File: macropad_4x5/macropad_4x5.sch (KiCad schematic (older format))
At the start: 41 parts

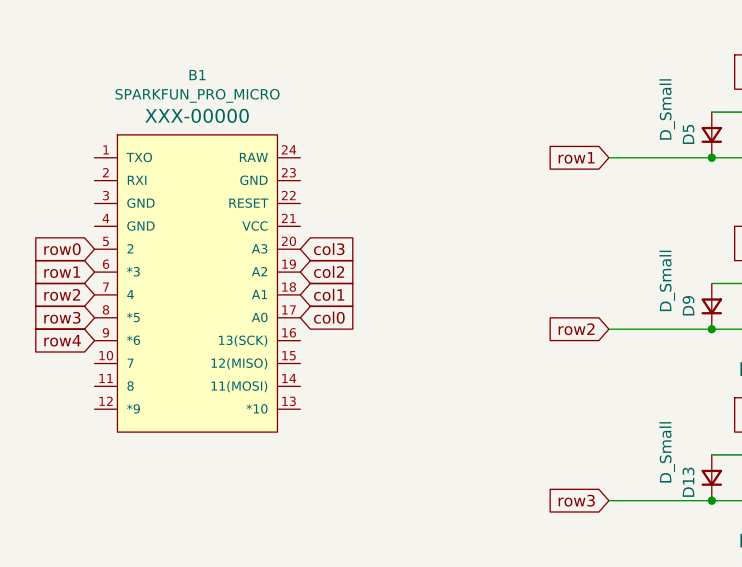
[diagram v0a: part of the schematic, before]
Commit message: Updated schematic and pcb routing
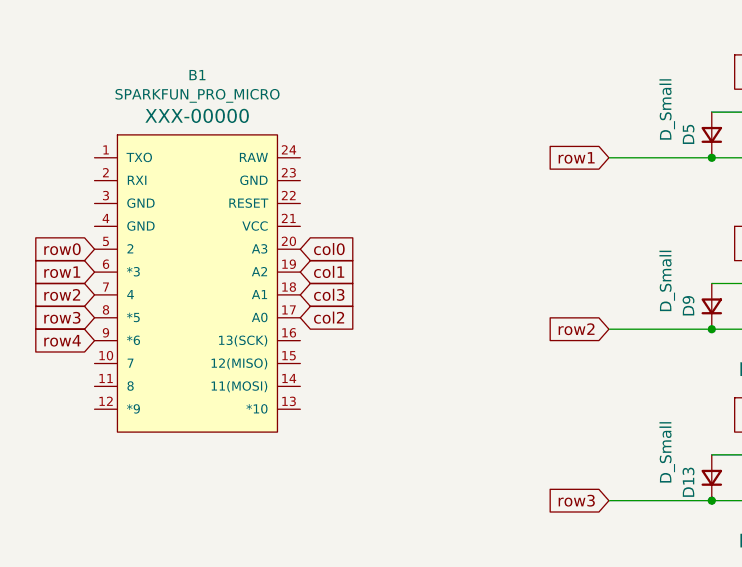
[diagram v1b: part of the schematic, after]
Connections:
- net col0: now also B1.20 (A3); no longer B1.17 (A0)
- net col1: now also B1.19 (A2); no longer B1.18 (A1)
- net col2: now also B1.17 (A0); no longer B1.19 (A2)
- net col3: now also B1.18 (A1); no longer B1.20 (A3)
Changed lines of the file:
@@
 Text GLabel 3450 4950 0    50   Input ~ 0
 row4
+Text GLabel 2100 3100 2    50   Input ~ 0
+col0
+Text GLabel 2100 3200 2    50   Input ~ 0
+col1
 Text GLabel 2100 3400 2    50   Input ~ 0
-col0
+col2
 Text GLabel 2100 3300 2    50   Input ~ 0
-col1
-Text GLabel 2100 3200 2    50   Input ~ 0
-col2
-Text GLabel 2100 3100 2    50   Input ~ 0
 col3
 Text GLabel 1200 3100 0    50   Input ~ 0
